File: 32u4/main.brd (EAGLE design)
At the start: 160 x 100 mm, 15 parts, among them U1 ATMEGA32U4-TQFP44, X1 MINI-USB-UX60A-MB-5ST

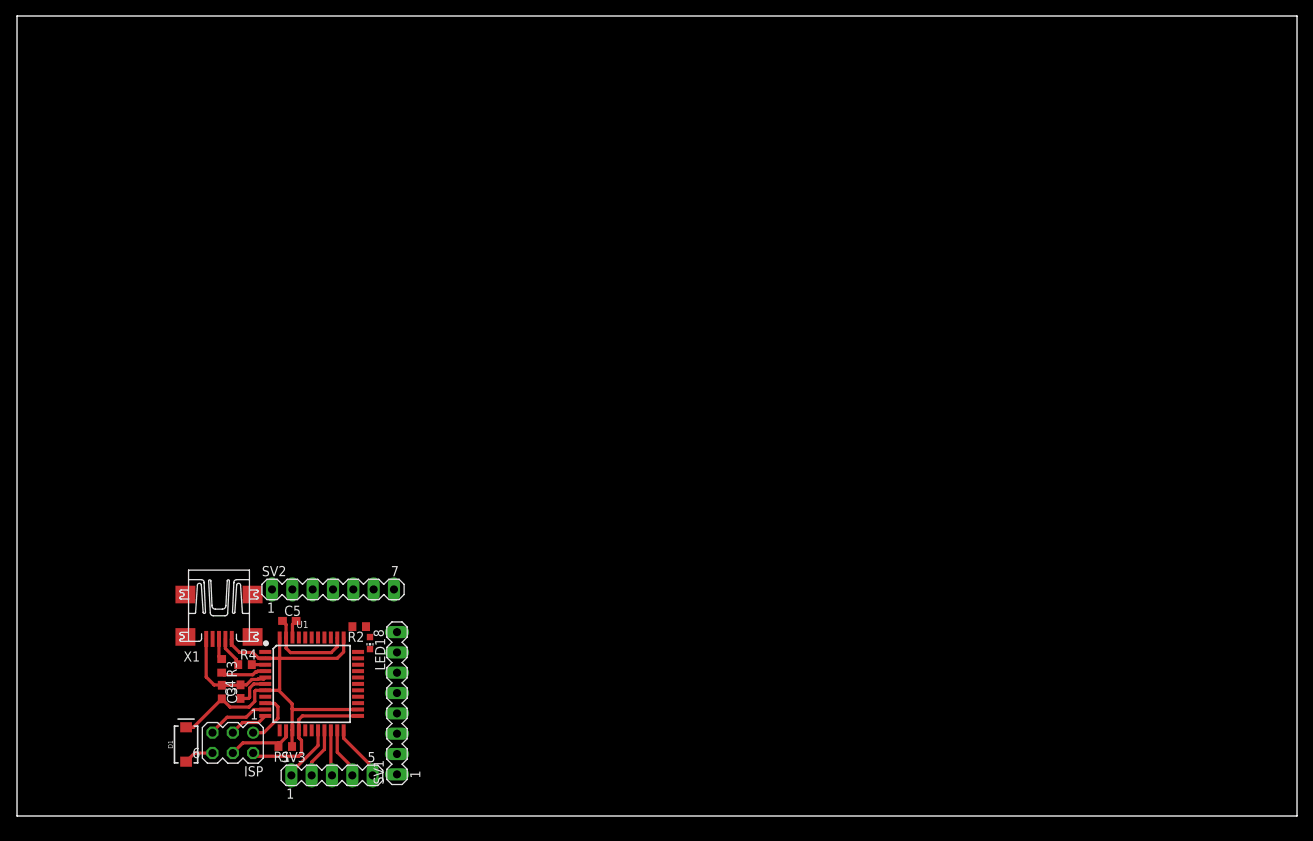
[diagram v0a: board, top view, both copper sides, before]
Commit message: sdfsdfsff
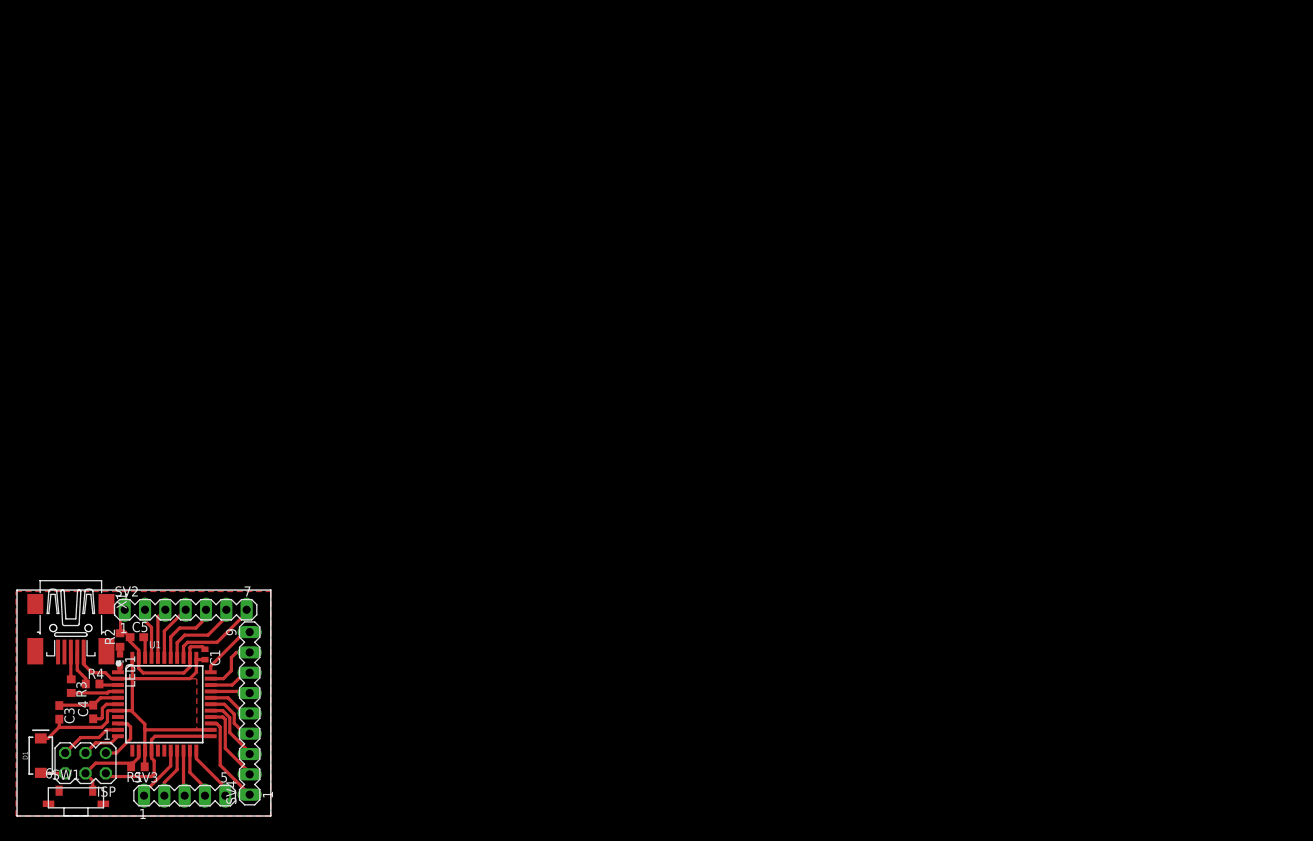
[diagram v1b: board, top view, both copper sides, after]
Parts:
- removed SV1: (no value), con-lstb:MA08-1
- added C1: 100n, rcl:C0402
- added SV4: (no value), con-lstb:MA09-1
- added SW1: TL3330, 7_segment_lib:TL3330
- X1: value MINI-USB-UX60A-MB-5ST -> MINI-USB-SCHIELD-32005-201; device con-hirose:UX60A-MB-5ST -> con-cypressindustries:32005-201
- moved LED1 31.3 mm to (12.9, 19.5)
- moved R2 29.9 mm to (12.9, 22.0), turned to 90 degrees
- moved C3 20.5 mm to (5.28, 13.0)
- moved R4 19.2 mm to (9.45, 16.5)
- moved C5 19.2 mm to (15.0, 22.4)
- moved R3 19.0 mm to (6.78, 16.2)
- moved C4 18.6 mm to (9.53, 13.0)
- moved ISP 18.6 mm to (8.56, 6.60)
- moved R1 18.6 mm to (15.1, 6.15)
- moved SV2 18.6 mm to (21.1, 25.8)
- moved SV3 18.6 mm to (21.0, 2.54)
- moved U1 18.6 mm to (18.4, 14.0)
- moved X1 18.5 mm to (6.73, 23.5)
- moved D1 18.2 mm to (2.97, 7.54)
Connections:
- removed net 2A: SV2.1, U1.1
- new net N$25: SV4.7, U1.31
- new net N$26: SV4.8, U1.32
- new net N$27: SV4.9, U1.33
- net GND: now also C1.1, R2.2, SV2.1, SW1.P$1@0, SW1.P$1@1, SW1.P$3, X1.M1, X1.M2, X1.M3, X1.M4
- net LED: now also U1.1
- net N$19: now also SV4.1; no longer SV1.1
- net N$20: now also SV4.2; no longer SV1.2
- net N$21: now also SV4.3; no longer SV1.3
- net N$22: now also SV4.4; no longer SV1.4
- net N$23: now also SV4.5; no longer SV1.5
- net N$24: now also SV4.6; no longer SV1.6
- net RST: now also SW1.P$4
- net VCC: now also C1.2; no longer R2.2
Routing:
- net N$18: track 0.00 -> 11.4 mm
- net N$19: track 0.00 -> 11.3 mm
- net N$17: track 0.00 -> 10.3 mm
- net N$20: track 0.00 -> 10.1 mm
- net N$16: track 0.00 -> 9.03 mm
- net N$21: track 0.00 -> 8.32 mm
- net N$27: track 0.00 -> 7.41 mm
- net N$26: track 0.00 -> 7.19 mm
- net N$15: track 0.00 -> 7.12 mm
- net N$22: track 0.00 -> 7.06 mm
- net N$14: track 0.00 -> 6.39 mm
- net N$13: track 0.00 -> 6.35 mm
- net N$23: track 0.00 -> 5.67 mm
- net N$25: track 0.00 -> 5.50 mm
- net N$24: track 0.00 -> 4.95 mm
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- added copper zone on layer 1, net GND
- added copper zone on layer 1, net VCC
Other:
- board size 160 x 100 mm -> 31.7 x 28.2 mm
